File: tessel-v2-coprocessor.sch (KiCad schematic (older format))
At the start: 46 parts, among them J401 CONN_02X05, J402 USB-micro-TH, J403 MODULE_HEADER, J404 MODULE_HEADER, J405 CONN_01X01, SW401 SW_PUSH, U401 SAMD21G14A-MU, X401 FC-135

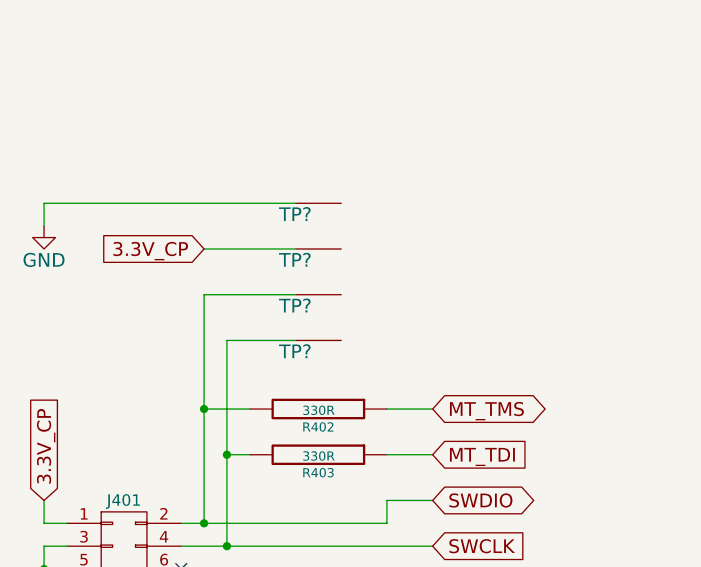
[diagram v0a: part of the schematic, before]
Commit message: annotated
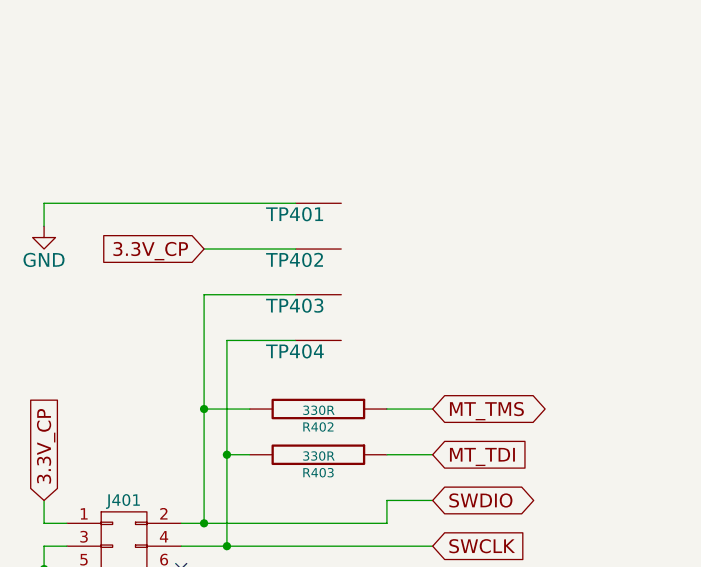
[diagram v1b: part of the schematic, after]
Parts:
- gave numbers to parts that had none: 4
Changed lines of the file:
@@
 $EndComp
 $Comp
-L GND #PWR0110
+L GND #PWR408
 U 1 1 548F9730
 P 4800 8050
-F 0 "#PWR0110" H 4800 8050 30  0001 C CNN
+F 0 "#PWR408" H 4800 8050 30  0001 C CNN
 F 1 "GND" H 4800 7980 30  0001 C CNN
 F 2 "" H 4800 8050 60  0000 C CNN
@@
 $EndComp
 $Comp
-L GND #PWR0111
+L GND #PWR410
 U 1 1 548F973F
 P 6000 8100
-F 0 "#PWR0111" H 6000 8100 30  0001 C CNN
+F 0 "#PWR410" H 6000 8100 30  0001 C CNN
 F 1 "GND" H 6000 8030 30  0001 C CNN
 F 2 "" H 6000 8100 60  0000 C CNN
@@
 VDDCORE
 $Comp
-L GND #PWR0112
+L GND #PWR417
 U 1 1 548FA205
 P 9400 3700
-F 0 "#PWR0112" H 9400 3700 30  0001 C CNN
+F 0 "#PWR417" H 9400 3700 30  0001 C CNN
 F 1 "GND" H 9400 3630 30  0001 C CNN
 F 2 "" H 9400 3700 60  0000 C CNN
@@
 $EndComp
 $Comp
-L GND #PWR0113
+L GND #PWR416
 U 1 1 548FBD70
 P 9000 3700
-F 0 "#PWR0113" H 9000 3700 30  0001 C CNN
+F 0 "#PWR416" H 9000 3700 30  0001 C CNN
 F 1 "GND" H 9000 3630 30  0001 C CNN
 F 2 "" H 9000 3700 60  0000 C CNN
@@
 $EndComp
 $Comp
-L GND #PWR0114
+L GND #PWR414
 U 1 1 548FBD83
 P 7500 3700
-F 0 "#PWR0114" H 7500 3700 30  0001 C CNN
+F 0 "#PWR414" H 7500 3700 30  0001 C CNN
 F 1 "GND" H 7500 3630 30  0001 C CNN
 F 2 "" H 7500 3700 60  0000 C CNN
@@
 $EndComp
 $Comp
-L GND #PWR0115
+L GND #PWR413
 U 1 1 548FBD8A
 P 7100 3700
-F 0 "#PWR0115" H 7100 3700 30  0001 C CNN
+F 0 "#PWR413" H 7100 3700 30  0001 C CNN
 F 1 "GND" H 7100 3630 30  0001 C CNN
 F 2 "" H 7100 3700 60  0000 C CNN
@@
 $EndComp
 $Comp
-L GND #PWR0116
+L GND #PWR412
 U 1 1 548FBD9D
 P 6700 3700
-F 0 "#PWR0116" H 6700 3700 30  0001 C CNN
+F 0 "#PWR412" H 6700 3700 30  0001 C CNN
 F 1 "GND" H 6700 3630 30  0001 C CNN
 F 2 "" H 6700 3700 60  0000 C CNN
@@
 $EndComp
 $Comp
-L GND #PWR0117
+L GND #PWR411
 U 1 1 548FBDA4
 P 6300 3700
-F 0 "#PWR0117" H 6300 3700 30  0001 C CNN
+F 0 "#PWR411" H 6300 3700 30  0001 C CNN
 F 1 "GND" H 6300 3630 30  0001 C CNN
 F 2 "" H 6300 3700 60  0000 C CNN
@@
 $EndComp
 $Comp
-L GND #PWR0118
+L GND #PWR409
 U 1 1 548FBDB7
 P 5900 3700
-F 0 "#PWR0118" H 5900 3700 30  0001 C CNN
+F 0 "#PWR409" H 5900 3700 30  0001 C CNN
 F 1 "GND" H 5900 3630 30  0001 C CNN
 F 2 "" H 5900 3700 60  0000 C CNN
@@
 $EndComp
 $Comp
-L GND #PWR0119
+L GND #PWR415
 U 1 1 548FD791
 P 8000 8100
-F 0 "#PWR0119" H 8000 8100 30  0001 C CNN
+F 0 "#PWR415" H 8000 8100 30  0001 C CNN
 F 1 "GND" H 8000 8030 30  0001 C CNN
 F 2 "" H 8000 8100 60  0000 C CNN
@@
 $EndComp
 $Comp
-L GND #PWR0120
+L GND #PWR422
 U 1 1 54E6B173
 P 14600 7700
-F 0 "#PWR0120" H 14600 7700 30  0001 C CNN
+F 0 "#PWR422" H 14600 7700 30  0001 C CNN
 F 1 "GND" H 14600 7630 30  0001 C CNN
 F 2 "" H 14600 7700 60  0000 C CNN
@@
 3.3V_CP
 $Comp
-L GND #PWR0121
+L GND #PWR419
 U 1 1 54E6B4A0
 P 13600 7700
-F 0 "#PWR0121" H 13600 7700 30  0001 C CNN
+F 0 "#PWR419" H 13600 7700 30  0001 C CNN
 F 1 "GND" H 13600 7630 30  0001 C CNN
 F 2 "" H 13600 7700 60  0000 C CNN
@@
 NoConn ~ 1400 6400
 $Comp
-L GND #PWR0122
+L GND #PWR403
 U 1 1 54E6D866
 P 1300 6600
-F 0 "#PWR0122" H 1300 6350 60  0001 C CNN
+F 0 "#PWR403" H 1300 6350 60  0001 C CNN
 F 1 "GND" H 1300 6450 60  0000 C CNN
 F 2 "" H 1300 6600 60  0000 C CNN
@@
 3.3V_PORTA
 $Comp
-L GND #PWR0123
+L GND #PWR420
 U 1 1 54E753B7
 P 14200 2400
-F 0 "#PWR0123" H 14200 2150 60  0001 C CNN
+F 0 "#PWR420" H 14200 2150 60  0001 C CNN
 F 1 "GND" H 14200 2250 60  0000 C CNN
 F 2 "" H 14200 2400 60  0000 C CNN
@@
 $EndComp
 $Comp
-L GND #PWR0124
+L GND #PWR421
 U 1 1 54E753CD
 P 14300 4200
-F 0 "#PWR0124" H 14300 3950 60  0001 C CNN
+F 0 "#PWR421" H 14300 3950 60  0001 C CNN
 F 1 "GND" H 14300 4050 60  0000 C CNN
 F 2 "" H 14300 4200 60  0000 C CNN
@@
 PORT_A_G3
 $Comp
-L +5V #PWR0125
+L +5V #PWR404
 U 1 1 54E79A0D
 P 2600 1400
-F 0 "#PWR0125" H 2600 1490 20  0001 C CNN
+F 0 "#PWR404" H 2600 1490 20  0001 C CNN
 F 1 "+5V" H 2600 1550 30  0000 C CNN
 F 2 "" H 2600 1400 60  0000 C CNN
@@
 $EndComp
 $Comp
-L GND #PWR0126
+L GND #PWR405
 U 1 1 54E79A13
 P 2600 2100
-F 0 "#PWR0126" H 2600 1850 60  0001 C CNN
+F 0 "#PWR405" H 2600 1850 60  0001 C CNN
 F 1 "GND" H 2600 1950 60  0000 C CNN
 F 2 "" H 2600 2100 60  0000 C CNN
@@
 $EndComp
 $Comp
-L GND #PWR0127
+L GND #PWR406
 U 1 1 54E79A19
 P 2900 2500
-F 0 "#PWR0127" H 2900 2250 60  0001 C CNN
+F 0 "#PWR406" H 2900 2250 60  0001 C CNN
 F 1 "GND" H 2900 2350 60  0000 C CNN
 F 2 "" H 2900 2500 60  0000 C CNN
@@
 $EndComp
 $Comp
-L GND #PWR0128
+L GND #PWR401
 U 1 1 54E79A1F
 P 1300 3100
-F 0 "#PWR0128" H 1300 2850 60  0001 C CNN
+F 0 "#PWR401" H 1300 2850 60  0001 C CNN
 F 1 "GND" H 1300 2950 60  0000 C CNN
 F 2 "" H 1300 3100 60  0000 C CNN
@@
 $EndComp
 $Comp
-L +5V #PWR0129
+L +5V #PWR407
 U 1 1 54E79A2D
 P 3800 2100
-F 0 "#PWR0129" H 3800 2190 20  0001 C CNN
+F 0 "#PWR407" H 3800 2190 20  0001 C CNN
 F 1 "+5V" H 3800 2250 30  0000 C CNN
 F 2 "" H 3800 2100 60  0000 C CNN
@@
 FLASH_~CS
 $Comp
-L GND #PWR0130
+L GND #PWR418
 U 1 1 54EE1D18
 P 11600 3500
-F 0 "#PWR0130" H 11600 3250 60  0001 C CNN
+F 0 "#PWR418" H 11600 3250 60  0001 C CNN
 F 1 "GND" H 11600 3350 60  0000 C CNN
 F 2 "" H 11600 3500 60  0000 C CNN
@@
 	13500 2100 13500 2200
 $Comp
-L TP TP?
+L TP TP403
 U 1 1 55076899
 P 2400 5000
-F 0 "TP?" H 2400 5050 60  0000 C CNN
+F 0 "TP403" H 2400 5050 60  0000 C CNN
 F 1 "TP" H 2400 4950 60  0001 C CNN
 F 2 "" H 2400 5000 60  0000 C CNN
@@
 $EndComp
 $Comp
-L TP TP?
+L TP TP404
 U 1 1 55076939
 P 2400 5200
-F 0 "TP?" H 2400 5250 60  0000 C CNN
+F 0 "TP404" H 2400 5250 60  0000 C CNN
 F 1 "TP" H 2400 5150 60  0001 C CNN
 F 2 "" H 2400 5200 60  0000 C CNN
@@
 3.3V_CP
 $Comp
-L TP TP?
+L TP TP402
 U 1 1 550772D3
 P 2400 4800
-F 0 "TP?" H 2400 4850 60  0000 C CNN
+F 0 "TP402" H 2400 4850 60  0000 C CNN
 F 1 "TP" H 2400 4750 60  0001 C CNN
 F 2 "" H 2400 4800 60  0000 C CNN
@@
 	2400 4800 2000 4800
 $Comp
-L GND #PWR?
+L GND #PWR402
 U 1 1 55077307
 P 1300 4700
-F 0 "#PWR?" H 1300 4450 60  0001 C CNN
+F 0 "#PWR402" H 1300 4450 60  0001 C CNN
 F 1 "GND" H 1300 4550 60  0000 C CNN
 F 2 "" H 1300 4700 60  0000 C CNN
@@
 $EndComp
 $Comp
-L TP TP?
+L TP TP401
 U 1 1 5507734C
 P 2400 4600
-F 0 "TP?" H 2400 4650 60  0000 C CNN
+F 0 "TP401" H 2400 4650 60  0000 C CNN
 F 1 "TP" H 2400 4550 60  0001 C CNN
 F 2 "" H 2400 4600 60  0000 C CNN

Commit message: netlist, etc.
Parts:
- TP401, TP402, TP403, TP404: footprint (none) -> tm-kicad-lib:Testpoint
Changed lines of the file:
@@
 $EndComp
 $Comp
-L GND #PWR408
+L GND #PWR0113
 U 1 1 548F9730
 P 4800 8050
-F 0 "#PWR408" H 4800 8050 30  0001 C CNN
+F 0 "#PWR0113" H 4800 8050 30  0001 C CNN
 F 1 "GND" H 4800 7980 30  0001 C CNN
 F 2 "" H 4800 8050 60  0000 C CNN
@@
 $EndComp
 $Comp
-L GND #PWR410
+L GND #PWR0114
 U 1 1 548F973F
 P 6000 8100
-F 0 "#PWR410" H 6000 8100 30  0001 C CNN
+F 0 "#PWR0114" H 6000 8100 30  0001 C CNN
 F 1 "GND" H 6000 8030 30  0001 C CNN
 F 2 "" H 6000 8100 60  0000 C CNN
@@
 VDDCORE
 $Comp
-L GND #PWR417
+L GND #PWR0115
 U 1 1 548FA205
 P 9400 3700
-F 0 "#PWR417" H 9400 3700 30  0001 C CNN
+F 0 "#PWR0115" H 9400 3700 30  0001 C CNN
 F 1 "GND" H 9400 3630 30  0001 C CNN
 F 2 "" H 9400 3700 60  0000 C CNN
@@
 $EndComp
 $Comp
-L GND #PWR416
+L GND #PWR0116
 U 1 1 548FBD70
 P 9000 3700
-F 0 "#PWR416" H 9000 3700 30  0001 C CNN
+F 0 "#PWR0116" H 9000 3700 30  0001 C CNN
 F 1 "GND" H 9000 3630 30  0001 C CNN
 F 2 "" H 9000 3700 60  0000 C CNN
@@
 $EndComp
 $Comp
-L GND #PWR414
+L GND #PWR0117
 U 1 1 548FBD83
 P 7500 3700
-F 0 "#PWR414" H 7500 3700 30  0001 C CNN
+F 0 "#PWR0117" H 7500 3700 30  0001 C CNN
 F 1 "GND" H 7500 3630 30  0001 C CNN
 F 2 "" H 7500 3700 60  0000 C CNN
@@
 $EndComp
 $Comp
-L GND #PWR413
+L GND #PWR0118
 U 1 1 548FBD8A
 P 7100 3700
-F 0 "#PWR413" H 7100 3700 30  0001 C CNN
+F 0 "#PWR0118" H 7100 3700 30  0001 C CNN
 F 1 "GND" H 7100 3630 30  0001 C CNN
 F 2 "" H 7100 3700 60  0000 C CNN
@@
 $EndComp
 $Comp
-L GND #PWR412
+L GND #PWR0119
 U 1 1 548FBD9D
 P 6700 3700
-F 0 "#PWR412" H 6700 3700 30  0001 C CNN
+F 0 "#PWR0119" H 6700 3700 30  0001 C CNN
 F 1 "GND" H 6700 3630 30  0001 C CNN
 F 2 "" H 6700 3700 60  0000 C CNN
@@
 $EndComp
 $Comp
-L GND #PWR411
+L GND #PWR0120
 U 1 1 548FBDA4
 P 6300 3700
-F 0 "#PWR411" H 6300 3700 30  0001 C CNN
+F 0 "#PWR0120" H 6300 3700 30  0001 C CNN
 F 1 "GND" H 6300 3630 30  0001 C CNN
 F 2 "" H 6300 3700 60  0000 C CNN
@@
 $EndComp
 $Comp
-L GND #PWR409
+L GND #PWR0121
 U 1 1 548FBDB7
 P 5900 3700
-F 0 "#PWR409" H 5900 3700 30  0001 C CNN
+F 0 "#PWR0121" H 5900 3700 30  0001 C CNN
 F 1 "GND" H 5900 3630 30  0001 C CNN
 F 2 "" H 5900 3700 60  0000 C CNN
@@
 $EndComp
 $Comp
-L GND #PWR415
+L GND #PWR0122
 U 1 1 548FD791
 P 8000 8100
-F 0 "#PWR415" H 8000 8100 30  0001 C CNN
+F 0 "#PWR0122" H 8000 8100 30  0001 C CNN
 F 1 "GND" H 8000 8030 30  0001 C CNN
 F 2 "" H 8000 8100 60  0000 C CNN
@@
 $EndComp
 $Comp
-L GND #PWR422
+L GND #PWR0123
 U 1 1 54E6B173
 P 14600 7700
-F 0 "#PWR422" H 14600 7700 30  0001 C CNN
+F 0 "#PWR0123" H 14600 7700 30  0001 C CNN
 F 1 "GND" H 14600 7630 30  0001 C CNN
 F 2 "" H 14600 7700 60  0000 C CNN
@@
 3.3V_CP
 $Comp
-L GND #PWR419
+L GND #PWR0124
 U 1 1 54E6B4A0
 P 13600 7700
-F 0 "#PWR419" H 13600 7700 30  0001 C CNN
+F 0 "#PWR0124" H 13600 7700 30  0001 C CNN
 F 1 "GND" H 13600 7630 30  0001 C CNN
 F 2 "" H 13600 7700 60  0000 C CNN
@@
 NoConn ~ 1400 6400
 $Comp
-L GND #PWR403
+L GND #PWR0125
 U 1 1 54E6D866
 P 1300 6600
-F 0 "#PWR403" H 1300 6350 60  0001 C CNN
+F 0 "#PWR0125" H 1300 6350 60  0001 C CNN
 F 1 "GND" H 1300 6450 60  0000 C CNN
 F 2 "" H 1300 6600 60  0000 C CNN
@@
 3.3V_PORTA
 $Comp
-L GND #PWR420
+L GND #PWR0126
 U 1 1 54E753B7
 P 14200 2400
-F 0 "#PWR420" H 14200 2150 60  0001 C CNN
+F 0 "#PWR0126" H 14200 2150 60  0001 C CNN
 F 1 "GND" H 14200 2250 60  0000 C CNN
 F 2 "" H 14200 2400 60  0000 C CNN
@@
 $EndComp
 $Comp
-L GND #PWR421
+L GND #PWR0127
 U 1 1 54E753CD
 P 14300 4200
-F 0 "#PWR421" H 14300 3950 60  0001 C CNN
+F 0 "#PWR0127" H 14300 3950 60  0001 C CNN
 F 1 "GND" H 14300 4050 60  0000 C CNN
 F 2 "" H 14300 4200 60  0000 C CNN
@@
 PORT_A_G3
 $Comp
-L +5V #PWR404
+L +5V #PWR0128
 U 1 1 54E79A0D
 P 2600 1400
-F 0 "#PWR404" H 2600 1490 20  0001 C CNN
+F 0 "#PWR0128" H 2600 1490 20  0001 C CNN
 F 1 "+5V" H 2600 1550 30  0000 C CNN
 F 2 "" H 2600 1400 60  0000 C CNN
@@
 $EndComp
 $Comp
-L GND #PWR405
+L GND #PWR0129
 U 1 1 54E79A13
 P 2600 2100
-F 0 "#PWR405" H 2600 1850 60  0001 C CNN
+F 0 "#PWR0129" H 2600 1850 60  0001 C CNN
 F 1 "GND" H 2600 1950 60  0000 C CNN
 F 2 "" H 2600 2100 60  0000 C CNN
@@
 $EndComp
 $Comp
-L GND #PWR406
+L GND #PWR0130
 U 1 1 54E79A19
 P 2900 2500
-F 0 "#PWR406" H 2900 2250 60  0001 C CNN
+F 0 "#PWR0130" H 2900 2250 60  0001 C CNN
 F 1 "GND" H 2900 2350 60  0000 C CNN
 F 2 "" H 2900 2500 60  0000 C CNN
@@
 $EndComp
 $Comp
-L GND #PWR401
+L GND #PWR0131
 U 1 1 54E79A1F
 P 1300 3100
-F 0 "#PWR401" H 1300 2850 60  0001 C CNN
+F 0 "#PWR0131" H 1300 2850 60  0001 C CNN
 F 1 "GND" H 1300 2950 60  0000 C CNN
 F 2 "" H 1300 3100 60  0000 C CNN
@@
 $EndComp
 $Comp
-L +5V #PWR407
+L +5V #PWR0132
 U 1 1 54E79A2D
 P 3800 2100
-F 0 "#PWR407" H 3800 2190 20  0001 C CNN
+F 0 "#PWR0132" H 3800 2190 20  0001 C CNN
 F 1 "+5V" H 3800 2250 30  0000 C CNN
 F 2 "" H 3800 2100 60  0000 C CNN
@@
 FLASH_~CS
 $Comp
-L GND #PWR418
+L GND #PWR0133
 U 1 1 54EE1D18
 P 11600 3500
-F 0 "#PWR418" H 11600 3250 60  0001 C CNN
+F 0 "#PWR0133" H 11600 3250 60  0001 C CNN
 F 1 "GND" H 11600 3350 60  0000 C CNN
 F 2 "" H 11600 3500 60  0000 C CNN
@@
 F 0 "TP403" H 2400 5050 60  0000 C CNN
 F 1 "TP" H 2400 4950 60  0001 C CNN
-F 2 "" H 2400 5000 60  0000 C CNN
+F 2 "tm-kicad-lib:Testpoint" H 2400 5000 60  0001 C CNN
 F 3 "" H 2400 5000 60  0000 C CNN
 	1    2400 5000
@@
 F 0 "TP404" H 2400 5250 60  0000 C CNN
 F 1 "TP" H 2400 5150 60  0001 C CNN
-F 2 "" H 2400 5200 60  0000 C CNN
+F 2 "tm-kicad-lib:Testpoint" H 2400 5200 60  0001 C CNN
 F 3 "" H 2400 5200 60  0000 C CNN
 	1    2400 5200
@@
 F 0 "TP402" H 2400 4850 60  0000 C CNN
 F 1 "TP" H 2400 4750 60  0001 C CNN
-F 2 "" H 2400 4800 60  0000 C CNN
+F 2 "tm-kicad-lib:Testpoint" H 2400 4800 60  0001 C CNN
 F 3 "" H 2400 4800 60  0000 C CNN
 	1    2400 4800
@@
 	2400 4800 2000 4800
 $Comp
-L GND #PWR402
+L GND #PWR0134
 U 1 1 55077307
 P 1300 4700
-F 0 "#PWR402" H 1300 4450 60  0001 C CNN
+F 0 "#PWR0134" H 1300 4450 60  0001 C CNN
 F 1 "GND" H 1300 4550 60  0000 C CNN
 F 2 "" H 1300 4700 60  0000 C CNN
@@
 F 0 "TP401" H 2400 4650 60  0000 C CNN
 F 1 "TP" H 2400 4550 60  0001 C CNN
-F 2 "" H 2400 4600 60  0000 C CNN
+F 2 "tm-kicad-lib:Testpoint" H 2400 4600 60  0001 C CNN
 F 3 "" H 2400 4600 60  0000 C CNN
 	1    2400 4600
